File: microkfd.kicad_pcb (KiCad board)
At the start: 2 copper layers, 60 x 20 mm, 48 parts, among them J1 USB_B_Micro, J2 AVR-ISP-6, J3 OLED, J4 AudioJack3, Q1 MMBT3904, Q2 MMBT3904, SW1 SW_UP, SW2 SW_DN, SW3 SW_ENT, U1 FT231XS, U2 ATmega328P-A, Y1 16MHz

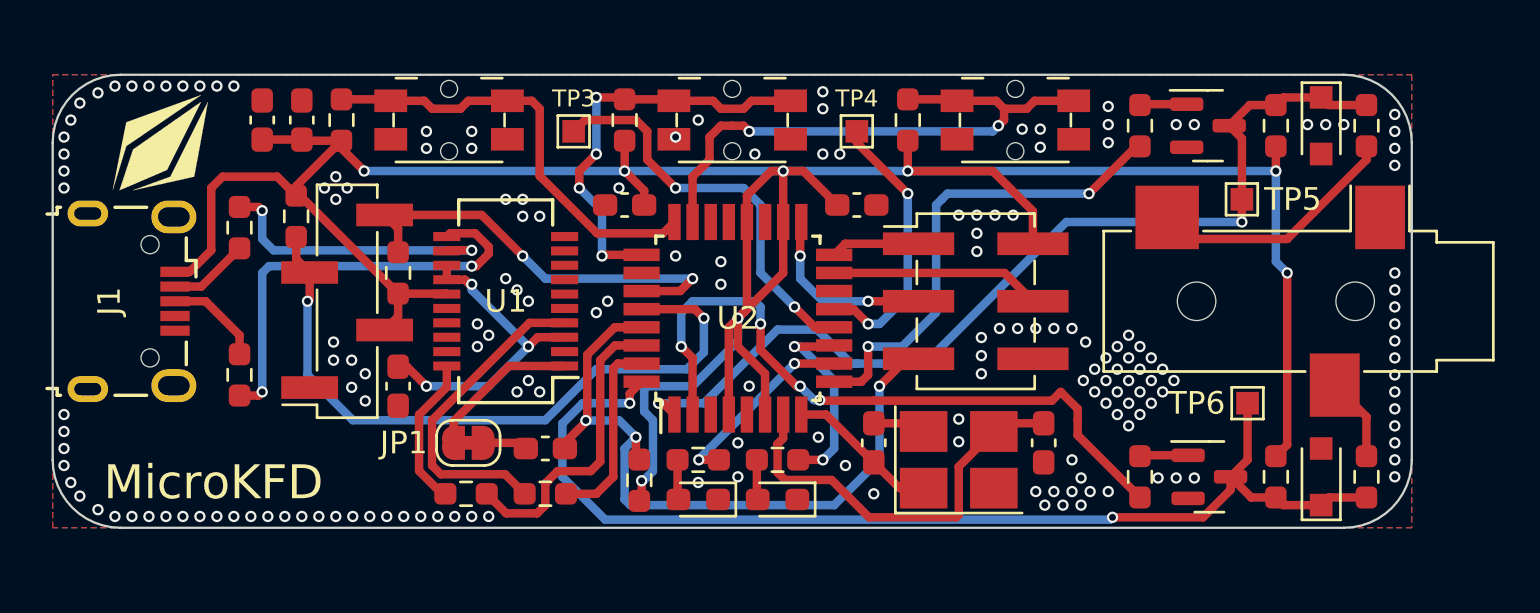
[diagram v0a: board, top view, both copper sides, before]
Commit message: finalized 328p design
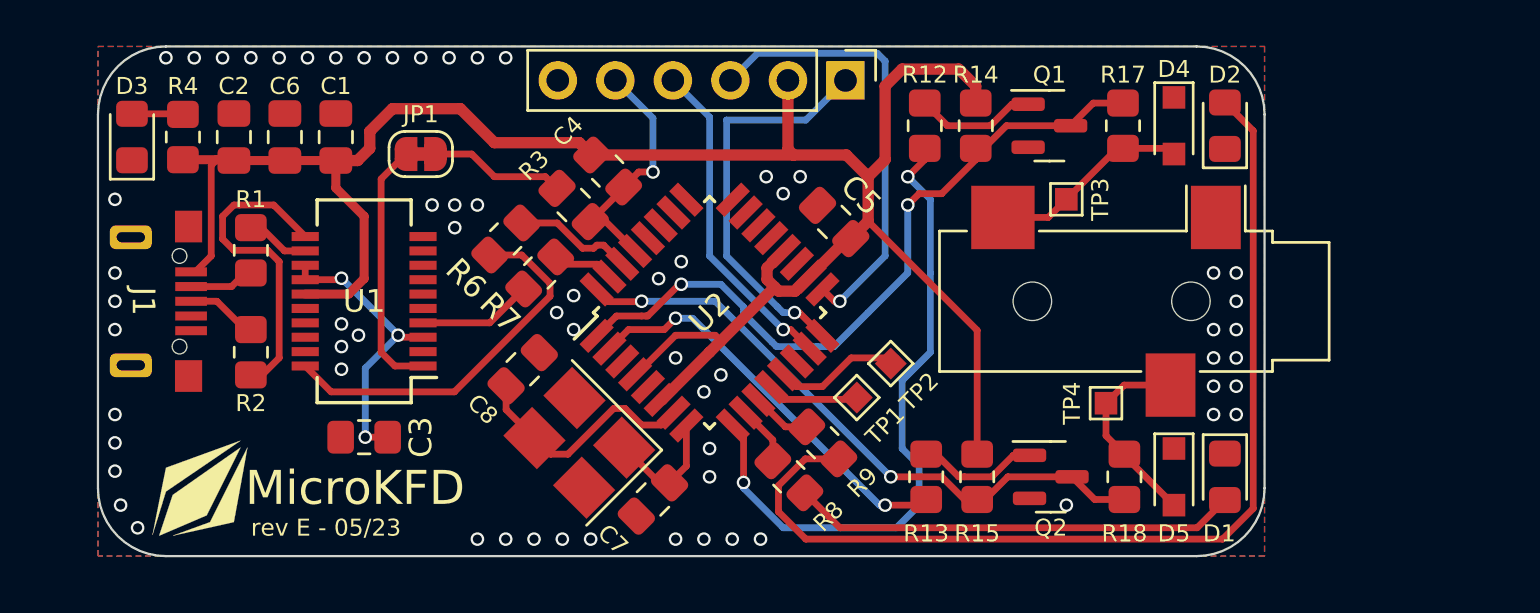
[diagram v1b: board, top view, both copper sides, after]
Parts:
- removed C10, C9: 10pF, Capacitor_SMD:C_0603_1608Metric_Pad1.08x0.95mm_HandSolder
- removed J3: OLED, Connector_PinHeader_2.54mm:PinHeader_1x04_P2.54mm_Vertical_SMD_Pin1Right
- removed R10, R11, R16, R5: 10k, Resistor_SMD:R_0603_1608Metric_Pad0.98x0.95mm_HandSolder
- removed SW1: SW_UP, Button_Switch_SMD:Panasonic_EVQPUM_EVQPUD
- removed SW2: SW_DN, Button_Switch_SMD:Panasonic_EVQPUM_EVQPUD
- removed SW3: SW_ENT, Button_Switch_SMD:Panasonic_EVQPUM_EVQPUD
- removed TP5: KFD_DATA, TestPoint:TestPoint_Pad_1.0x1.0mm
- removed TP6: KFD_SENSE, TestPoint:TestPoint_Pad_1.0x1.0mm
- added C1: 0.1uF, Capacitor_SMD:C_0805_2012Metric_Pad1.18x1.45mm_HandSolder, F.Cu at (107.5, 92.8)
- added C3: 0.1uF, Capacitor_SMD:C_0805_2012Metric_Pad1.18x1.45mm_HandSolder, F.Cu at (108.8, 106.0)
- added D5: 6.3V, Diode_SMD:D_SOD-323_HandSoldering, F.Cu at (144.5, 107.8)
- added TP1: GPIO1, TestPoint:TestPoint_Pad_1.0x1.0mm, F.Cu at (130.5, 104.2)
- added TP2: GPIO2, TestPoint:TestPoint_Pad_1.0x1.0mm, F.Cu at (132.0, 102.8)
- C2: value 0.1uF -> 10uF; footprint Capacitor_SMD:C_0603_1608Metric_Pad1.08x0.95mm_HandSolder -> Capacitor_SMD:C_0805_2012Metric_Pad1.18x1.45mm_HandSolder
- C4: value 10uF -> 0.1uF; footprint Capacitor_SMD:C_0603_1608Metric_Pad1.08x0.95mm_HandSolder -> Capacitor_SMD:C_0805_2012Metric_Pad1.18x1.45mm_HandSolder
- C5, C6: footprint Capacitor_SMD:C_0603_1608Metric_Pad1.08x0.95mm_HandSolder -> Capacitor_SMD:C_0805_2012Metric_Pad1.18x1.45mm_HandSolder
- C7, C8: value 0.1uF -> 8pF; footprint Capacitor_SMD:C_0603_1608Metric_Pad1.08x0.95mm_HandSolder -> Capacitor_SMD:C_0805_2012Metric_Pad1.18x1.45mm_HandSolder
- D1, D2: footprint LED_SMD:LED_0603_1608Metric_Pad1.05x0.95mm_HandSolder -> LED_SMD:LED_0805_2012Metric_Pad1.15x1.40mm_HandSolder
- D3: value 6.3V -> D_PWR; footprint Diode_SMD:D_SOD-323_HandSoldering -> LED_SMD:LED_0805_2012Metric_Pad1.15x1.40mm_HandSolder
- J1: footprint Connector_USB:USB_Micro-B_Wuerth_629105150521 -> lcsc-comps:U254-051N-4BH83-F1B
- J2: footprint Connector_PinHeader_2.54mm:PinHeader_2x03_P2.54mm_Vertical_SMD -> Connector_PinHeader_2.54mm:PinHeader_1x06_P2.54mm_Vertical
- R1, R12, R13, R14, R15, R17, R18, R2, R3, R6, R7, R8, R9: footprint Resistor_SMD:R_0603_1608Metric_Pad0.98x0.95mm_HandSolder -> Resistor_SMD:R_0805_2012Metric_Pad1.20x1.40mm_HandSolder
- R4: value 10k -> 1k; footprint Resistor_SMD:R_0603_1608Metric_Pad0.98x0.95mm_HandSolder -> Resistor_SMD:R_0805_2012Metric_Pad1.20x1.40mm_HandSolder
- TP3: value GPIO1 -> KFD_DATA
- TP4: value GPIO2 -> KFD_SENSE
- moved D3 52.5 mm to (98.5, 92.8), turned to 90 degrees
- moved D2 25.7 mm to (146.8, 92.2), turned to 90 degrees
- moved D1 23.3 mm to (146.8, 107.8), turned to -90 degrees
- moved TP3 22.0 mm to (139.8, 95.5)
- moved C5 20.6 mm to (129.5, 96.5), turned to -45 degrees
- moved C6 17.9 mm to (105.2, 92.8), turned to -90 degrees
- moved D4 16.8 mm to (144.5, 92.2), turned to -90 degrees
- moved Y1 16.8 mm to (118.2, 106.2), turned to 135 degrees
- moved C8 16.4 mm to (115.8, 103.0), turned to -135 degrees
- moved TP4 16.3 mm to (141.5, 104.5)
- moved G*** 15.4 mm to (101.5, 108.2)
- moved C4 14.3 mm to (118.0, 95.8), turned to -45 degrees
- moved R3 13.7 mm to (119.5, 94.2), turned to 135 degrees
- moved R14 13.2 mm to (135.8, 92.2), turned to 90 degrees
- moved R15 13.2 mm to (135.8, 107.8)
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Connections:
- C4 pad 1: +5V -> Net-(C4-Pad1)
- C4 pad 2: GND -> ~{RESET}
- C5 pad 1: Net-(C5-Pad1) -> GND
- C5 pad 2: GND -> +5V
- C6 pad 1: Net-(C6-Pad1) -> GND
- C6 pad 2: ~{RESET} -> +5V
- C7 pad 2: +5V -> Net-(C7-Pad2)
- C8 pad 2: +5V -> Net-(C8-Pad2)
- D3 pad 1: TWI_D_RX -> GND
- D3 pad 2: GND -> Net-(D3-Pad2)
- D4 pad 1: TWI_S_RX -> GND
- D4 pad 2: GND -> KFD_DATA
- JP1 pad 2: Net-(C6-Pad1) -> Net-(C4-Pad1)
- R4 pad 1: SDA -> Net-(D3-Pad2)
- TP3 pad 1: GPIO1 -> KFD_DATA
- TP4 pad 1: GPIO2 -> KFD_SENSE
- U1 pad 13: Net-(C5-Pad1) -> Net-(C3-Pad1)
- U1 pad 14: Net-(C5-Pad1) -> Net-(C3-Pad1)
- U1 pad 3: Net-(C5-Pad1) -> Net-(C3-Pad1)
- U2 pad 23: A0 -> unconnected-(U2-Pad23)
- U2 pad 24: A1 -> unconnected-(U2-Pad24)
- U2 pad 25: A2 -> unconnected-(U2-Pad25)
- U2 pad 27: SDA -> unconnected-(U2-Pad27)
- U2 pad 28: SCL -> unconnected-(U2-Pad28)
- U2 pad 7: Net-(C10-Pad2) -> Net-(C8-Pad2)
- U2 pad 8: Net-(C9-Pad2) -> Net-(C7-Pad2)
- Y1 pad 1: Net-(C9-Pad2) -> Net-(C7-Pad2)
- Y1 pad 3: Net-(C10-Pad2) -> Net-(C8-Pad2)
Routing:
- net Net-(D2-Pad2): track 1.77 -> 44.8 mm
- net +5V: track 133.0 -> 93.6 mm, vias 8 -> 0
- net SCL: track 30.4 -> 0.00 mm, vias 2 -> 0
- net A0: track 25.7 -> 0.00 mm, vias 2 -> 0
- net TWI_S_RX: track 48.5 -> 28.0 mm
- net ~{RESET}: track 30.8 -> 10.9 mm, vias 3 -> 1
- net A1: track 19.4 -> 0.00 mm
- net SDA: track 19.1 -> 0.00 mm, vias 2 -> 0
- net A2: track 18.4 -> 0.00 mm, vias 4 -> 0
- net Net-(C10-Pad2): track 18.2 -> 0.00 mm
- net Net-(D1-Pad2): track 1.77 -> 19.7 mm
- net Net-(C5-Pad1): track 14.2 -> 0.00 mm, vias 3 -> 0
- net GPIO1: track 18.0 -> 4.04 mm, vias 2 -> 0
- net MISO: track 3.93 -> 17.7 mm, vias 0 -> 1
- net Net-(C3-Pad1): track 0.00 -> 13.0 mm, vias 0 -> 3
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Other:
- board size 60 x 20 mm -> 51.5 x 22.5 mm
- board text added: "rev E - 05/23"
- board text removed: "rev E - 01/23"
